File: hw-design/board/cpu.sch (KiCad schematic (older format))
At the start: 11 parts, among them P10 CPU_RESET, P3 CHAIN, P9 SWD, U3 LPC11U24FBD48/401, Y1 12MHz

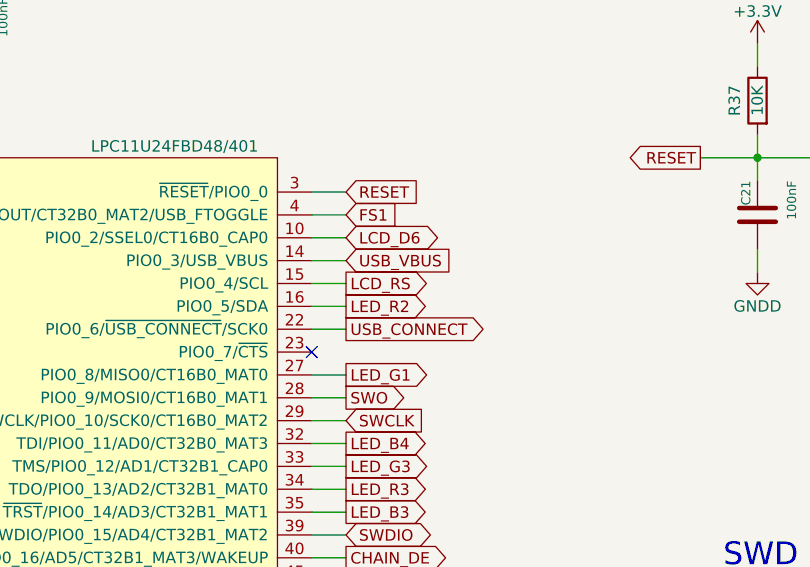
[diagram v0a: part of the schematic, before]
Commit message: only trigger isp when usb is connected
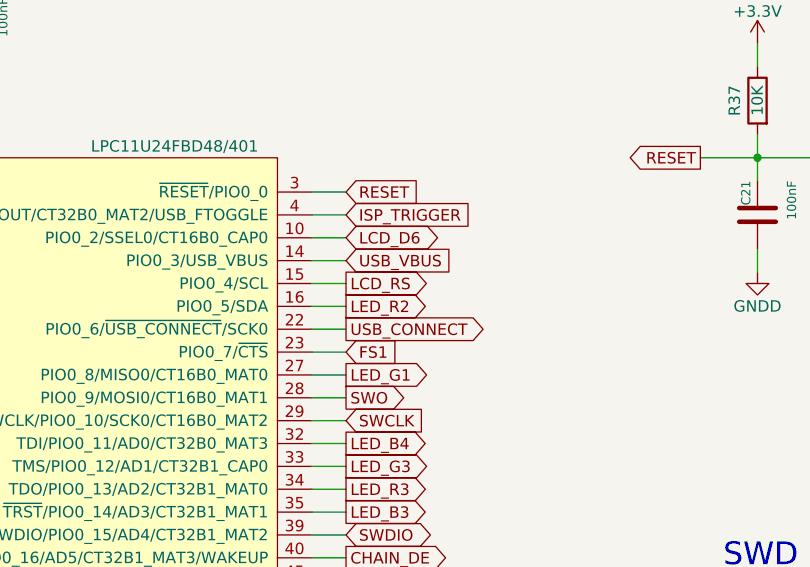
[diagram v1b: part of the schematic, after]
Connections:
- net labels added: ISP_TRIGGER
- wire segments 79 -> 80
- no-connect marks 8 -> 7
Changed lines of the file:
@@
 Text GLabel 7500 3450 2    50   Output ~ 0
 SWO
-Text GLabel 7500 2650 2    50   Input ~ 0
+Text GLabel 7500 3250 2    50   Input ~ 0
 FS1
 Text GLabel 3600 3950 0    50   Input ~ 0
@@
 LED_B4
 NoConn ~ 3750 3350
-NoConn ~ 7350 3250
 NoConn ~ 3750 3650
 $Comp
@@
 	7500 3450 7350 3450
 Wire Wire Line
-	7350 2650 7500 2650
+	7350 3250 7500 3250
 Wire Wire Line
 	3600 3950 3750 3950
@@
 NoConn ~ 3750 3050
 NoConn ~ 7350 4850
+Text GLabel 7500 2650 2    50   Input ~ 0
+ISP_TRIGGER
+Wire Wire Line
+	7350 2650 7500 2650
 $EndSCHEMATC
